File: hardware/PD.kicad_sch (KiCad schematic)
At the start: 11 parts, among them J7 USB_C_Receptacle_USB2.0_14P, U3 CH224K

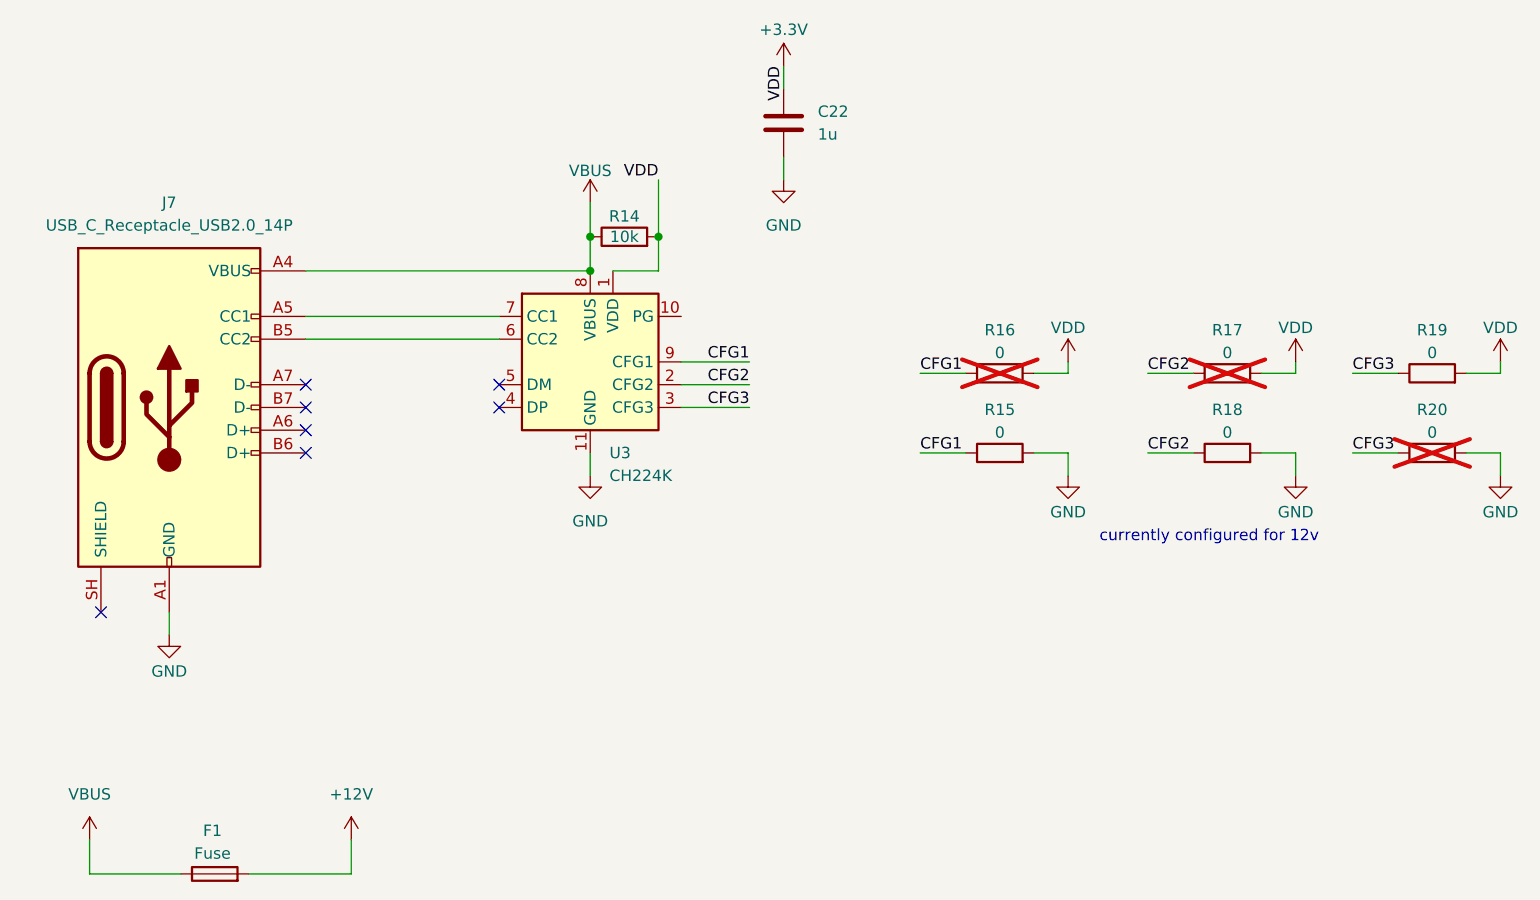
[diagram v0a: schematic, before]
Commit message: matthew review or get touched
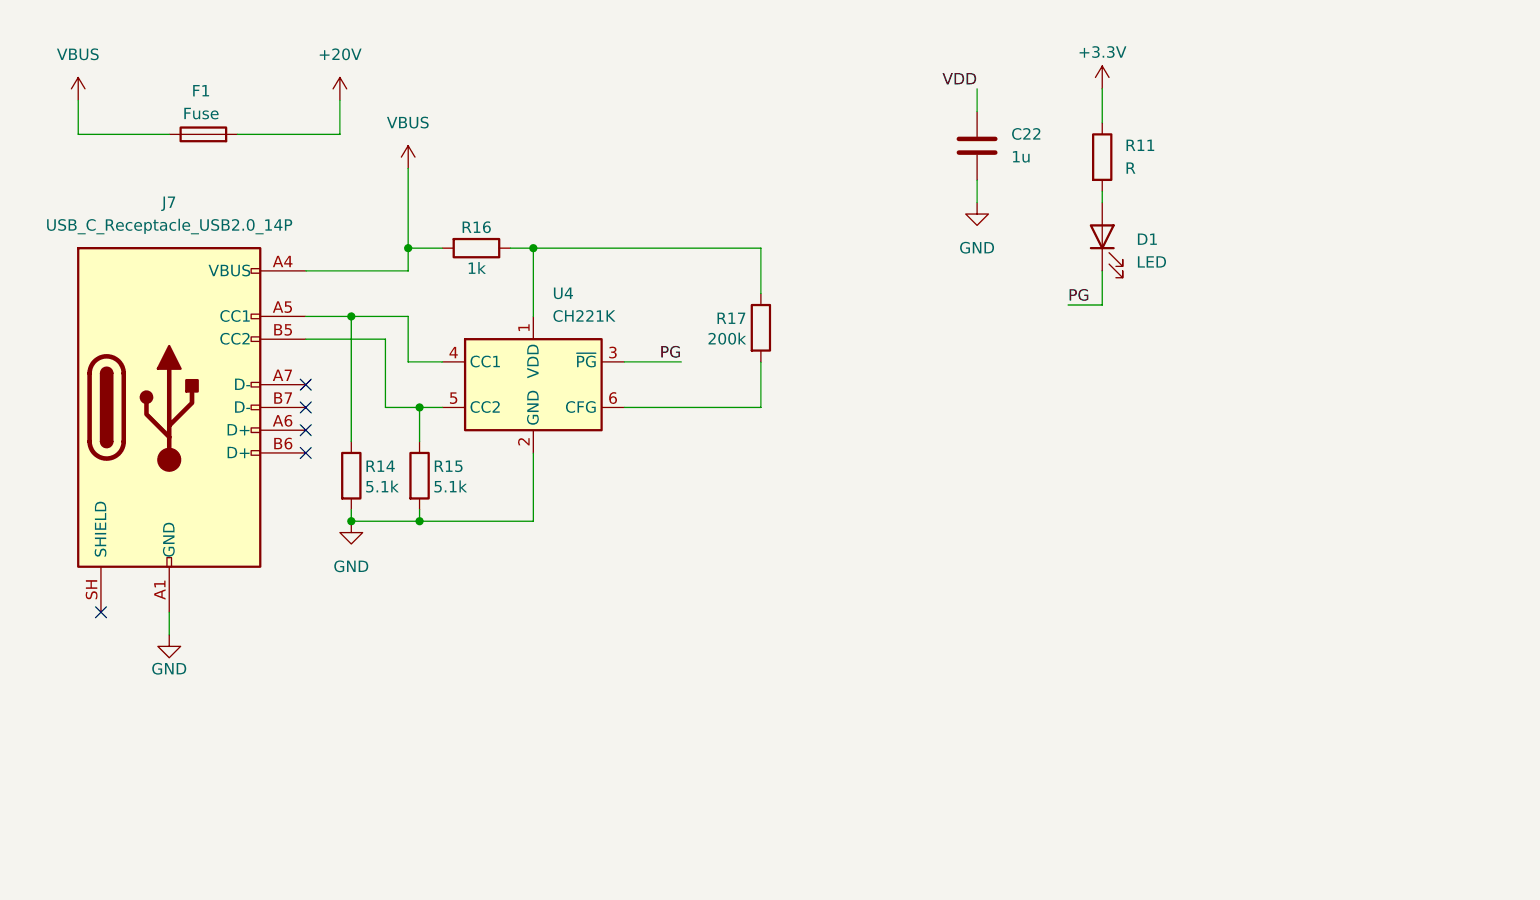
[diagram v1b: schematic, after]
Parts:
- removed R18, R19, R20: 0, symbol Device:R
- removed U3: CH224K, Package_SO:SSOP-10-1EP_3.9x4.9mm_P1mm_EP2.1x3.3mm, symbol Interface_USB:CH224K
- added D1: LED, symbol Device:LED
- added R11: R, symbol Device:R
- added U4: CH221K, Package_TO_SOT_SMD:SOT-23-6, symbol Interface_USB:CH221K
- R14: value 10k -> 5.1k
- R15: value 0 -> 5.1k
- R16: value 0 -> 1k; now fitted
- R17: value 0 -> 200k; now fitted
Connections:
- net CFG2 is gone; now on an unnamed net: R17.1
- net +3.3V: now also R11.1; no longer C22.1, R14.2, R16.2, R17.2
- net GND: now also R14.2, U4.2 (GND)
- net VBUS: now also R16.2; no longer R14.1
- net at J7.A5 (CC1): now also R14.1, U4.4 (CC1)
- net at J7.B5 (CC2): now also R15.1, U4.5 (CC2)
- net +12V renamed +20V
- net CFG1: no longer names the net of R16.1
- net CFG1: now also U4.1 (VDD); no longer R15.1
- new net: D1.2 (A), R11.2
- new net: R17.2, U4.6 (CFG)
- new net PG: D1.1 (K), U4.3 (~{PG})
- new net VDD: C22.1
- no-connect marks 7 -> 5
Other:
- note removed: "currently configured for 12v"
- moved on the sheet: C22, F1
